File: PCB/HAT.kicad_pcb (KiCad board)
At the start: 2 copper layers, 99.3 x 98.9 mm, 103 parts, among them J1 Conn_01x02_Pin, J10 Conn_01x24_Socket, J11 Conn_01x24_Pin, J12 Conn_01x02_Pin, J13 Conn_01x02_Pin, J14 Conn_01x02_Pin, J15 Conn_01x02_Pin, J2 Conn_01x02_Pin, J3 Conn_01x01_Pin, J4 Conn_01x02_Pin, J5 Conn_01x10_Pin, J6 MICROXNJ, J7 Conn_01x01_Pin, J8 Conn_01x24_Pin, J9 Conn_01x24_Socket, Q1 AO3401A, Q2 LBSS84LT1G, Q3 LBSS84LT1G, Q4 BSS138, Q5 BSS138, Q6 BSS138, Q7 BSS138, Q8 LM317AG-TN3-R, U1 TP4056, U2 XC6206P, U3 OP07, U4 VL6180, U6 CAT24C256, U7 CH340C, Y1 C252310

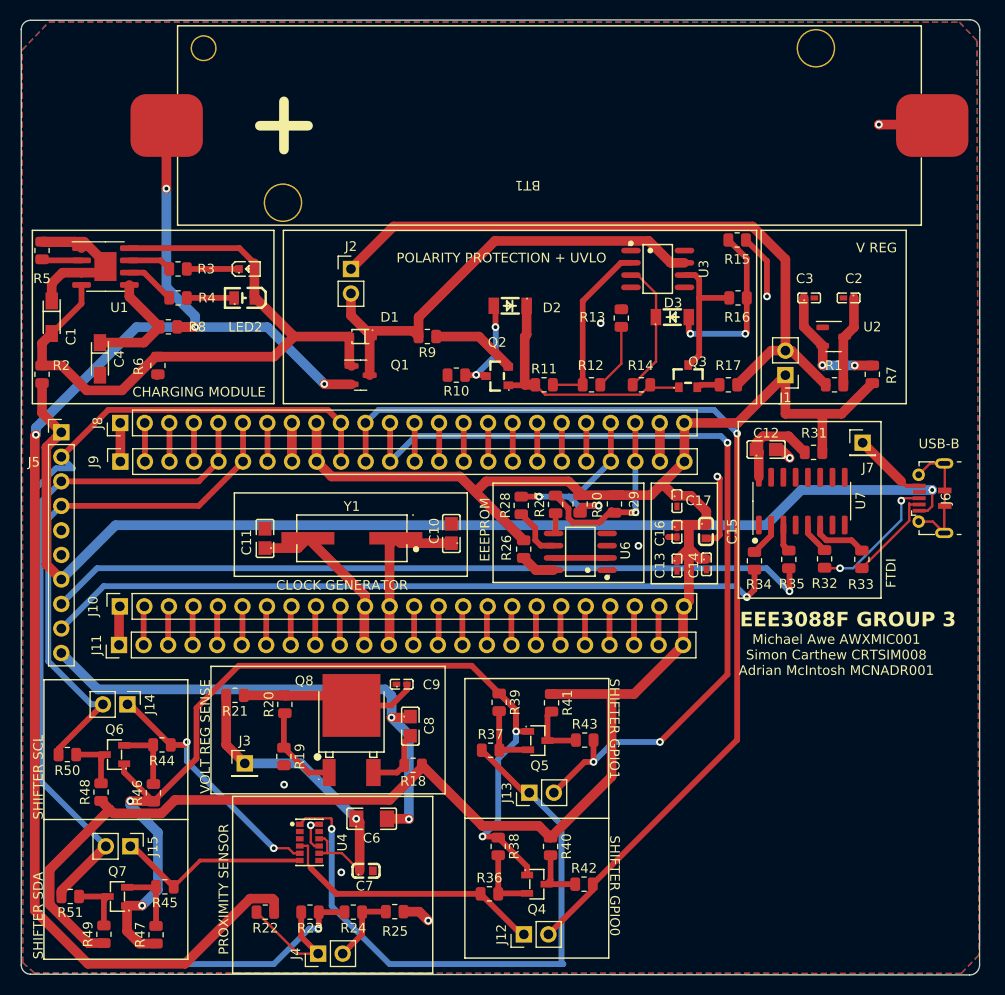
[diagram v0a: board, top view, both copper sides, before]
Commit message: Final Fixes
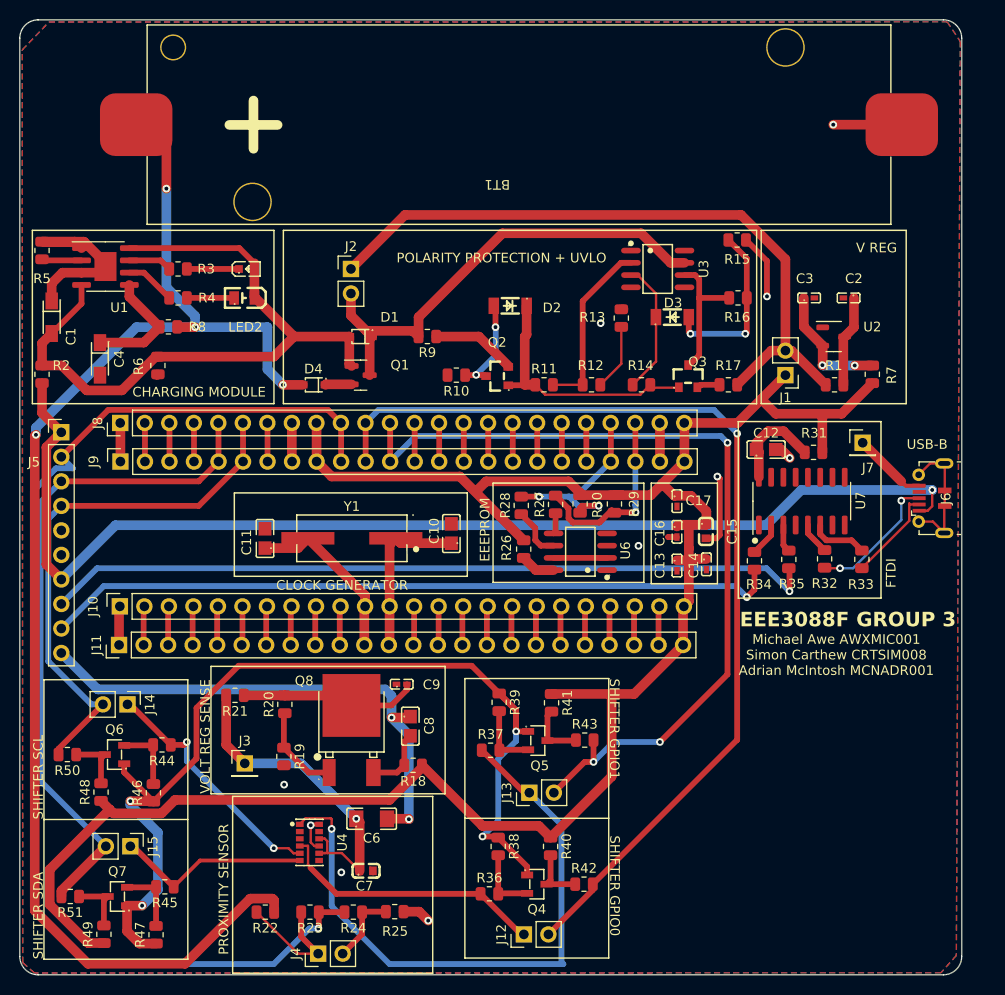
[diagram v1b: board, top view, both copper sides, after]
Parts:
- added D4: D_Schottky, JLC_Diodes:SOD-323_L1.8-W1.3-LS2.5-RD, F.Cu at (126.8, 84.7)
- moved BT1 3.16 mm to (148.0, 57.2)
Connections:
- Q1 pad 2: /Power Module/V_BAT+ -> Net-(D4-K)
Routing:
- net Net-(D4-K): track 0.00 -> 2.73 mm
- net /Power Module/V_BAT+: track 144.7 -> 142.2 mm
- net /MicroController_Interfacing/3V3: track 220.9 -> 219.1 mm
- net GND: track 126.1 -> 127.6 mm
- net /Power Module/UVLO_3V3: track 69.8 -> 70.8 mm
- net /Power Module/CHRG_OUT: track 48.9 -> 49.5 mm
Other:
- board size 99.3 x 98.9 mm -> 97.6 x 98.9 mm
